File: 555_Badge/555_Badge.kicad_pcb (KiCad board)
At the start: 2 copper layers, 96.5 x 98.3 mm, 15 parts, among them Q1 2N3904, U1 7555

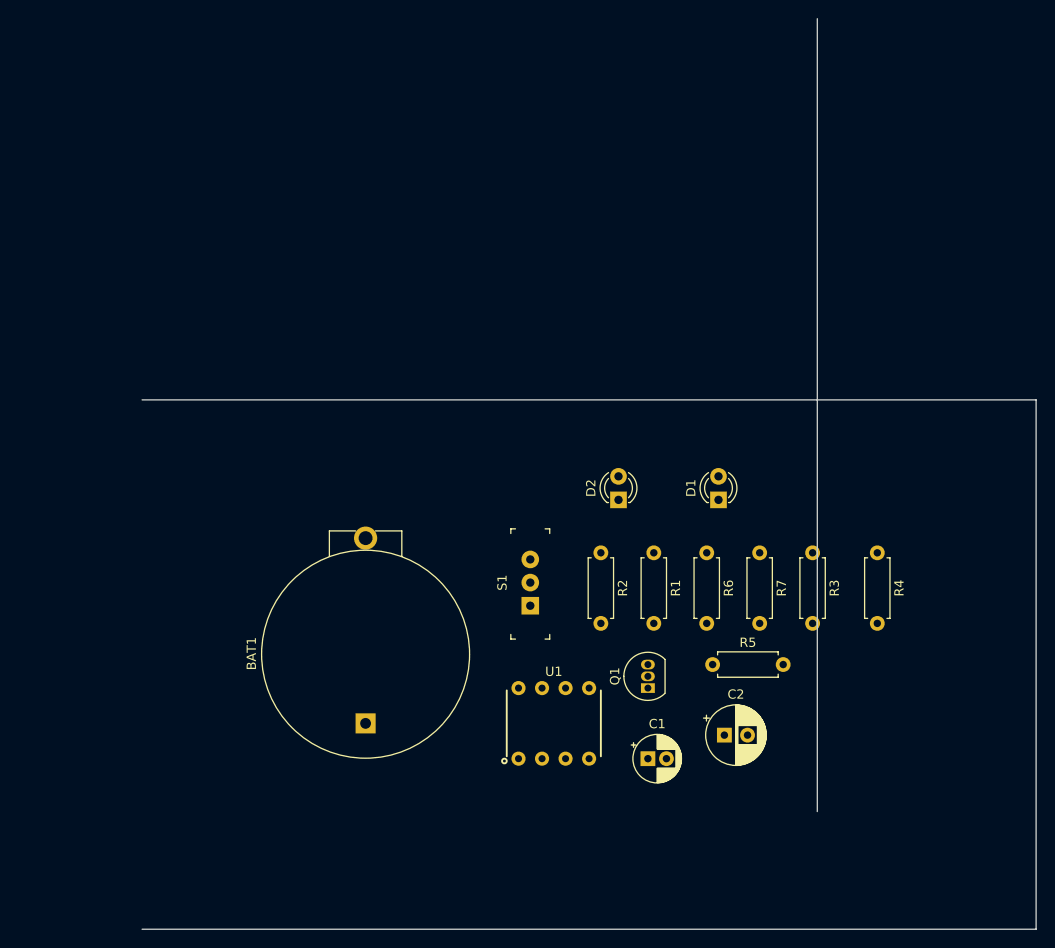
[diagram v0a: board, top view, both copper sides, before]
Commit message: Place completed
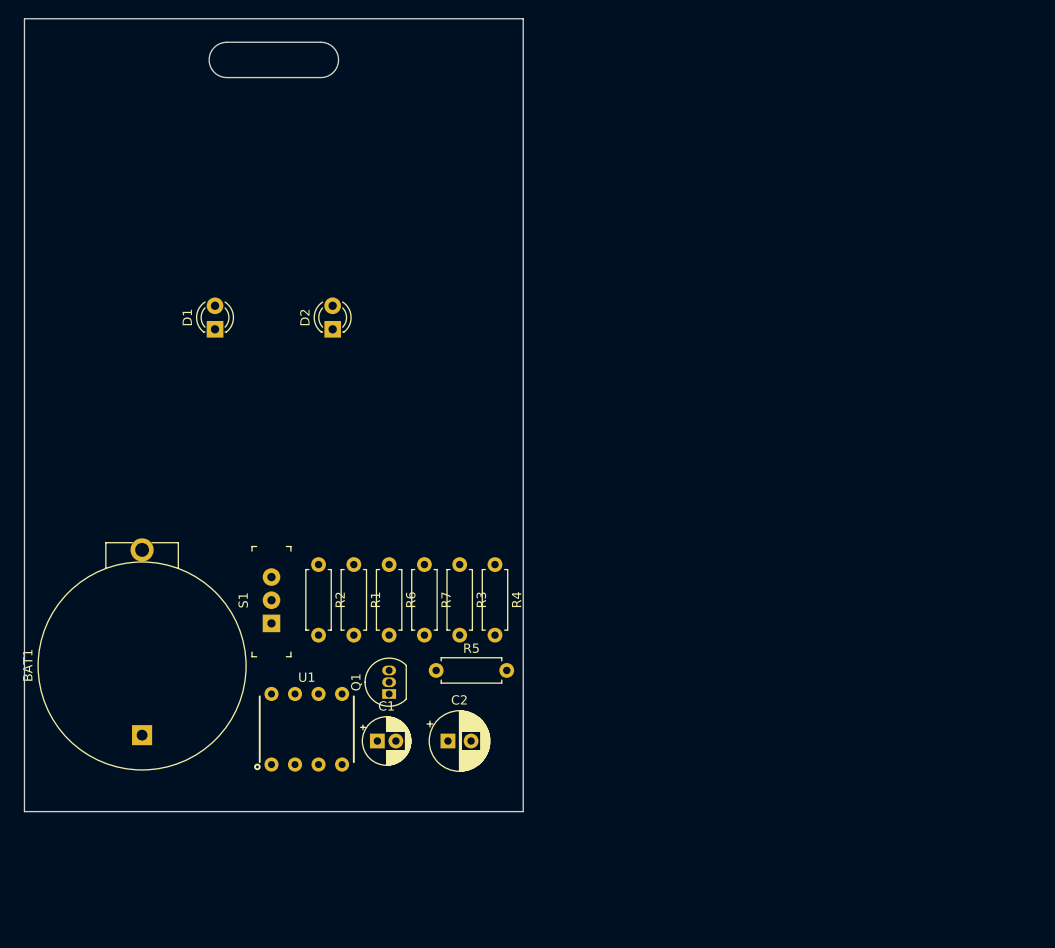
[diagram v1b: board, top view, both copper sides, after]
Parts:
- moved D1 57.4 mm to (147.6, 74.9)
- moved R4 41.3 mm to (177.8, 100.3)
- moved R3 38.1 mm to (174.0, 100.3)
- moved R7 36.2 mm to (170.2, 100.3)
- moved D2 35.9 mm to (160.3, 74.9)
- moved R6 34.3 mm to (166.4, 100.3)
- moved R1 32.4 mm to (162.6, 100.3)
- moved R2 30.5 mm to (158.8, 100.3)
- moved C2 29.9 mm to (172.7, 119.4)
- moved R5 29.9 mm to (171.4, 111.8)
- moved C1 29.3 mm to (165.1, 119.4)
- moved S1 28.0 mm to (153.7, 106.7)
- moved Q1 27.9 mm to (166.4, 114.3)
- moved U1 26.7 mm to (157.5, 118.1)
- moved BAT1 24.2 mm to (139.7, 118.7)
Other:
- board size 96.5 x 98.3 mm -> 53.8 x 85.6 mm
